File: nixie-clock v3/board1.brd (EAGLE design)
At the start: 139.7 x 50.8 mm, 29 parts, among them IC1 74HC573N, IC2 74HC573N, IC3 74HC573N, IC4 74HC573N, IC5 74HC573N, IC6 74HC573N

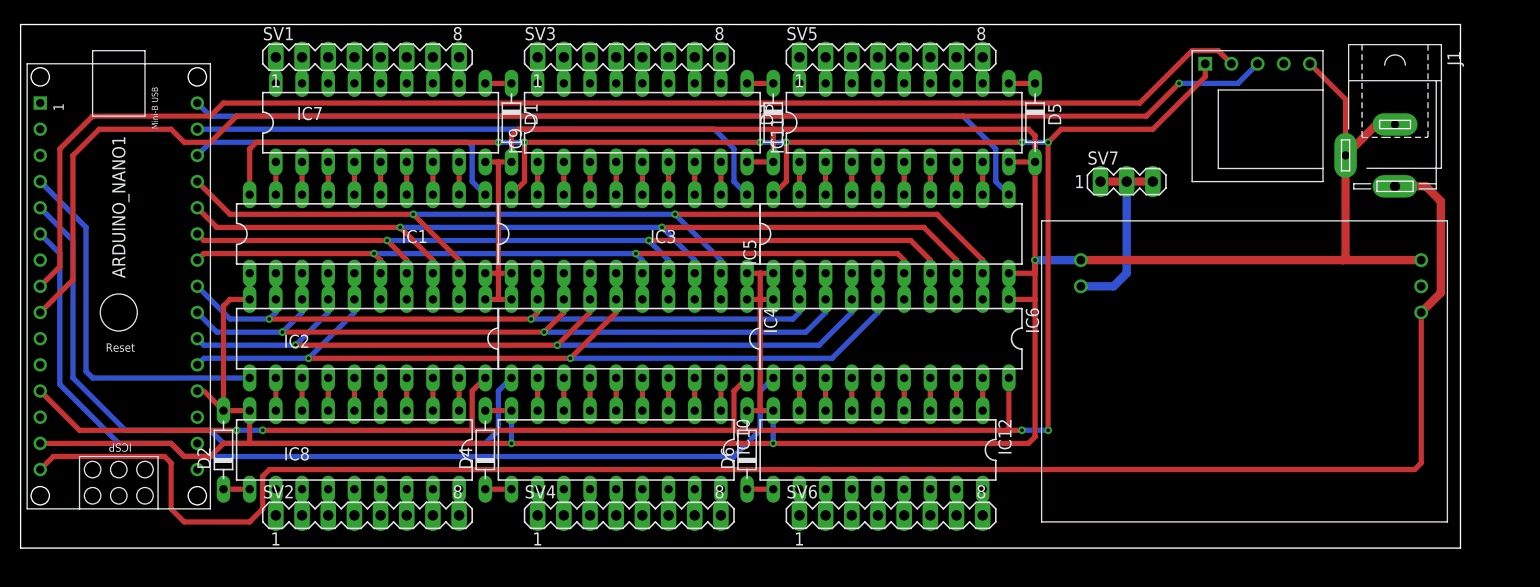
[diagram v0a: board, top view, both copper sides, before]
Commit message: lots of board progress
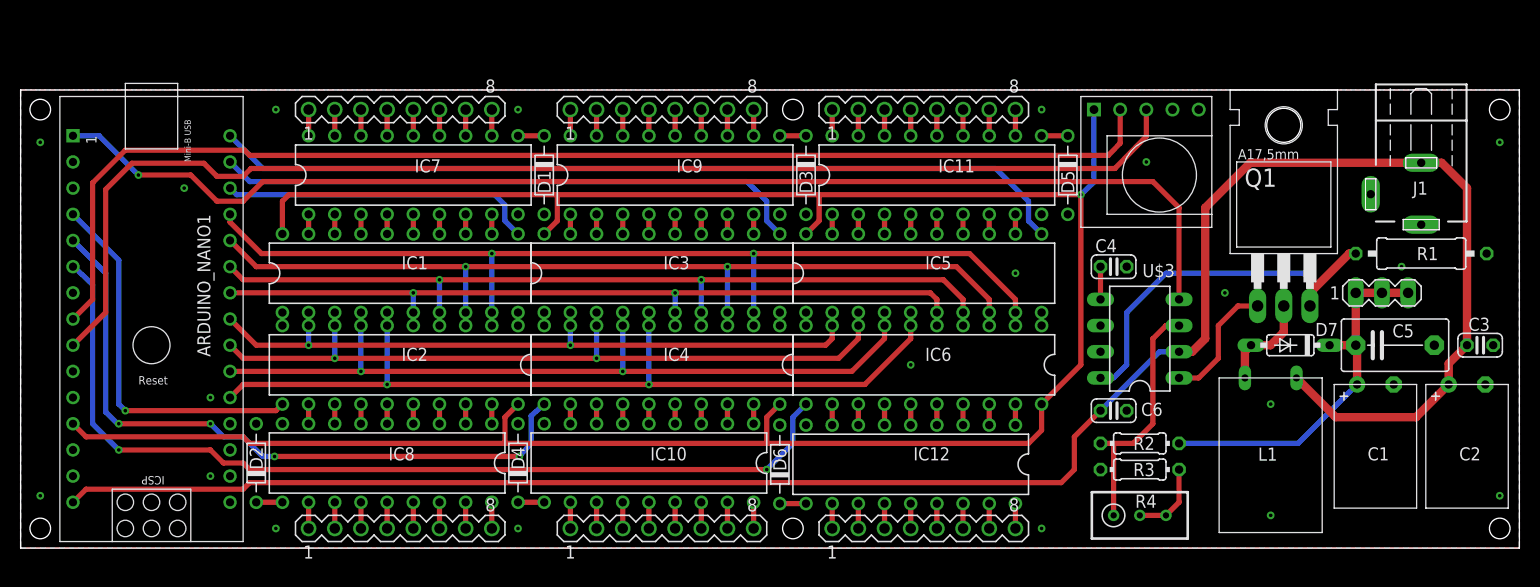
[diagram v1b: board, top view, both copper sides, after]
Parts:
- removed U$2: MAX1771_NIXIE_MODULE, random:MAX1771_NIXIE_MODULE
- added C1, C2: (no value), resistor-mod:E3,5-8
- added C3, C4, C6: (no value), resistor:C025-024X044
- added C5: (no value), capacitor-wima:C7.5B5
- added D7: (no value), diode:DO35-7
- added L1: (no value), inductor-neosid-mod:BS11
- added Q1: IRF620, transistor-fet:TO220
- added R1: (no value), resistor:0309/12
- added R2: 1M5, rcl:0204/7
- added R3: 10k, rcl:0204/7
- added R4: 5k, resistor:RTRIM3296W
- added U$3: MAX1771, maxim:DIL08
- D1, D2, D3, D4, D5, D6: device diode:D-7.5 -> diode-mod:D-7.5
- IC1, IC2, IC3, IC4, IC5, IC6: device 74xx-eu:DIL20 -> 74xx-eu-mod:DIL20
- IC10, IC11, IC12, IC7, IC8, IC9: device uln-udn:DIL18 -> uln-udn-mod:DIL18
- J1: value (none) -> NEB21R; device con-jack:SPC4077 -> con-lumberg:NEB21R
- SV1, SV2, SV3, SV4, SV5, SV6: device con-lstb:MA08-1 -> con-lstb-mod:MA08-1
- moved SV7 27.0 mm to (132.1, 24.8)
- moved U$1 11.7 mm to (109.2, 37.5)
- moved IC11 5.99 mm to (88.9, 36.2)
- moved IC7 5.99 mm to (38.1, 36.2)
- moved D1 5.99 mm to (50.8, 36.2)
- moved D3 5.99 mm to (76.2, 36.2)
- moved D5 5.99 mm to (101.6, 36.2)
- moved IC9 5.99 mm to (63.5, 36.2)
- moved SV1 5.99 mm to (36.8, 42.5)
- moved SV3 5.99 mm to (62.2, 42.5)
- moved SV5 5.99 mm to (87.6, 42.5)
- moved IC1 4.96 mm to (36.8, 26.7)
- moved IC3 4.96 mm to (62.2, 26.7)
- moved IC5 4.96 mm to (87.6, 26.7)
- moved ARDUINO_NANO1 4.49 mm to (12.7, 19.7)
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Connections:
- removed net N$101: SV7.1, SV7.2, SV7.3, U$2.5
- new net HV: C1.+, C5.1, D7.C, R2.2, SV7.1, SV7.2, SV7.3
- new net N$105: C4.1, U$3.5
- new net N$107: Q1.1, U$3.1
- new net N$109: D7.A, L1.2, Q1.2
- new net N$110: Q1.3, R1.2, U$3.8
- new net N$112: R2.1, R4.1, U$3.3
- new net N$113: R3.2, R4.2, R4.3
- new net SHDN: ARDUINO_NANO1.1, U$3.4
- net +12V: now also C2.+, C3.1, C6.1, L1.1, U$3.2; no longer U$2.1
- net GND: now also C1.-, C2.-, C3.2, C4.2, C5.2, C6.2, R1.1, R3.1, U$3.6, U$3.7; no longer U$2.3, U$2.4
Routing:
- net GND: track 335.0 -> 0.00 mm, vias 3 -> 20
- net SHDN: track 0.00 -> 120.7 mm, vias 0 -> 1
- net N$110: track 0.00 -> 37.6 mm
- net HV: track 0.00 -> 36.2 mm
- net VCC: track 256.1 -> 226.8 mm, vias 10 -> 1
- net N$112: track 0.00 -> 24.2 mm
- net +12V: track 175.2 -> 196.7 mm
- net N$101: track 18.9 -> 0.00 mm
- net N$97: track 132.3 -> 119.0 mm
- net N$99: track 136.2 -> 123.2 mm, vias 1 -> 0
- net N$107: track 0.00 -> 12.4 mm
- net N$109: track 0.00 -> 9.66 mm
- net N$113: track 0.00 -> 7.51 mm
- net D4: track 92.1 -> 84.9 mm
- net D8: track 103.4 -> 96.6 mm
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- added copper zone on layer 1, net GND
- added copper zone on layer 16, net GND
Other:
- board size 139.7 x 50.8 mm -> 145.4 x 44.5 mm
